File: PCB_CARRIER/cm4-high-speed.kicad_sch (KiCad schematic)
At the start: 1 part

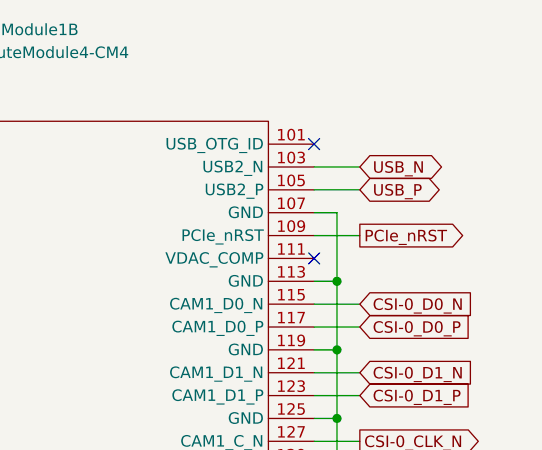
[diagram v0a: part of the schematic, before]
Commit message: fixed some label names for routing
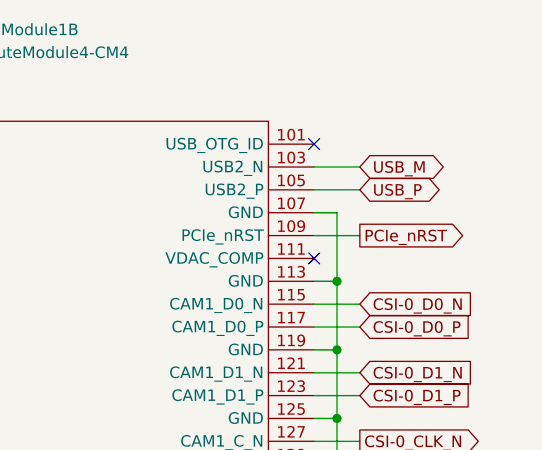
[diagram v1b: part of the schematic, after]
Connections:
- net USB_N renamed USB_M
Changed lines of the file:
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@@
 		)
 	)
-	(global_label "USB_N"
+	(global_label "USB_M"
 		(shape bidirectional)
 		(at 165.1 38.1 0)
@@
 		)
 		(property "Intersheetrefs" "${INTERSHEET_REFS}"
-			(at 175.3044 38.1 0)
+			(at 175.4253 38.1 0)
 			(effects
 				(font

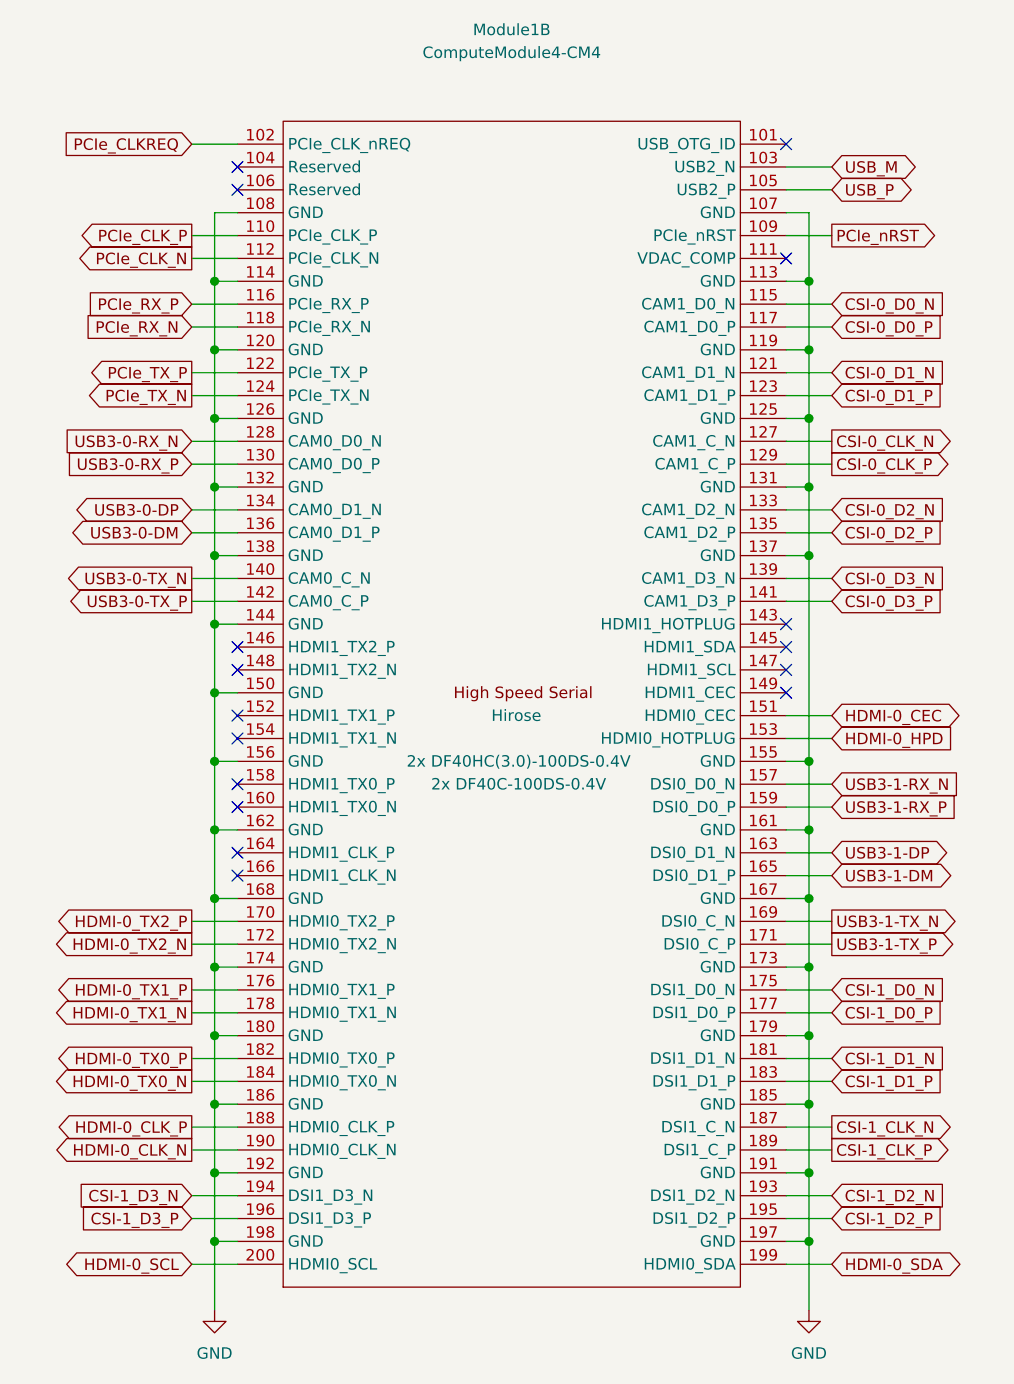
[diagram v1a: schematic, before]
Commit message: renaming all labels to use N instead of M
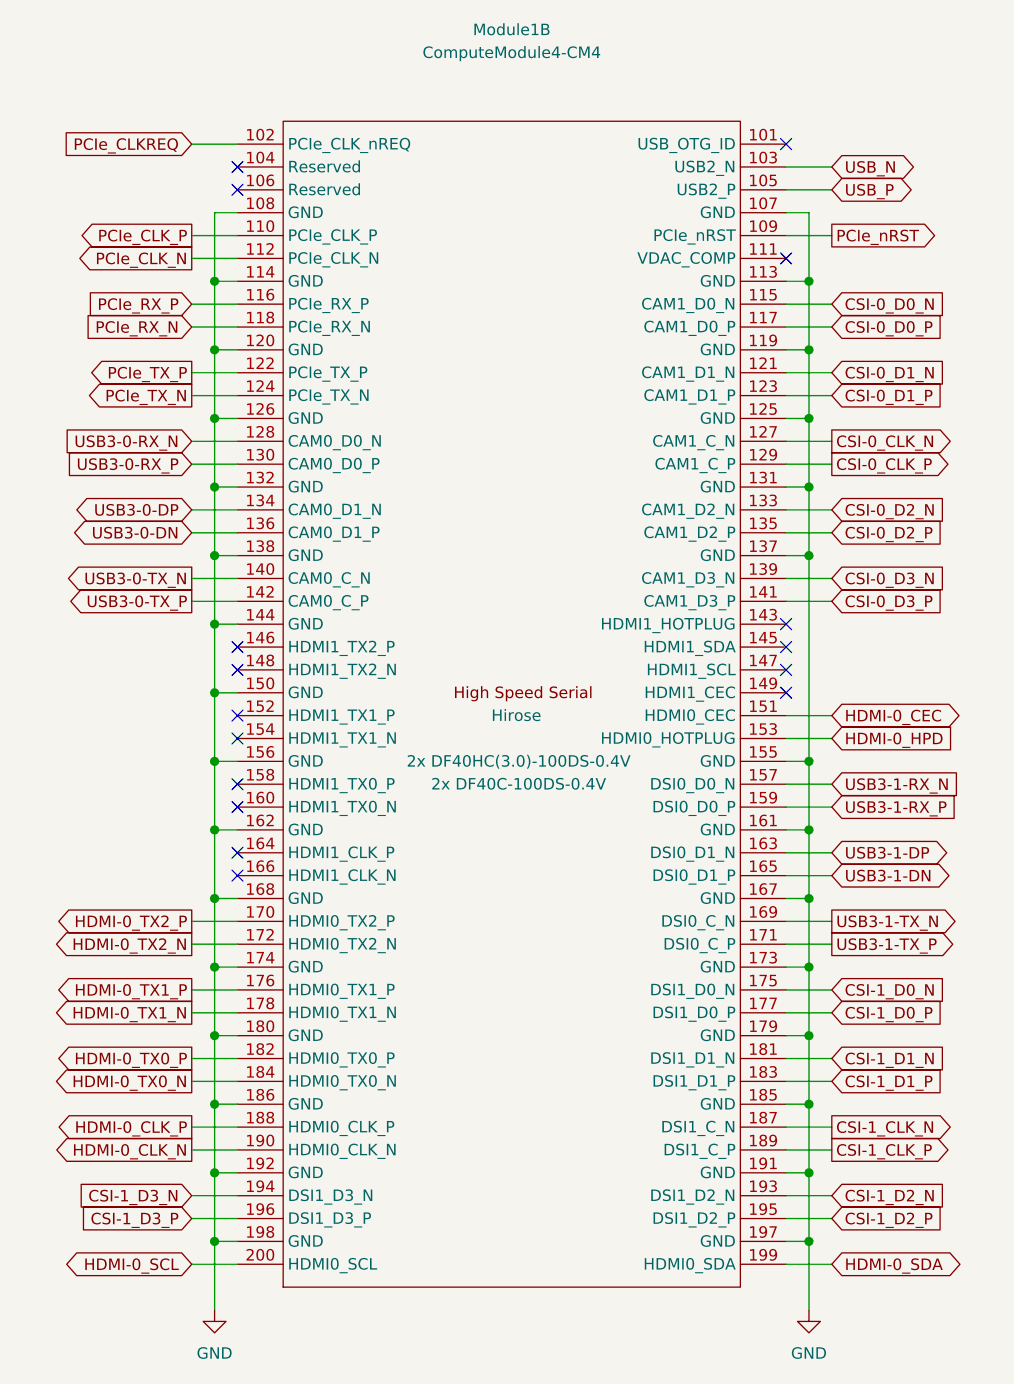
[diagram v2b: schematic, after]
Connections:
- net USB3-0-DM renamed USB3-0-DN
- net USB3-1-DM renamed USB3-1-DN
- net USB_M renamed USB_N
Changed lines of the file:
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@@
 		)
 	)
-	(global_label "USB3-1-DM"
+	(global_label "USB3-1-DN"
 		(shape bidirectional)
 		(at 165.1 116.84 0)
@@
 		)
 		(property "Intersheetrefs" "${INTERSHEET_REFS}"
-			(at 181.2915 116.84 0)
+			(at 181.1706 116.84 0)
 			(effects
 				(font
@@
 		)
 	)
-	(global_label "USB3-0-DM"
+	(global_label "USB3-0-DN"
 		(shape bidirectional)
 		(at 93.98 78.74 180)
@@
 		)
 		(property "Intersheetrefs" "${INTERSHEET_REFS}"
-			(at 77.7885 78.74 0)
+			(at 77.9094 78.74 0)
 			(effects
 				(font
@@
 		)
 	)
-	(global_label "USB_M"
+	(global_label "USB_N"
 		(shape bidirectional)
 		(at 165.1 38.1 0)
@@
 		)
 		(property "Intersheetrefs" "${INTERSHEET_REFS}"
-			(at 175.4253 38.1 0)
-			(effects
-				(font
+			(at 175.3044 38.1 0)
+			(effects
+				(font
